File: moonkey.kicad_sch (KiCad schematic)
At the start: 35 parts, among them SW1 SW_Push, SW10 SW_Push, SW11 SW_Push, SW12 SW_Push, SW13 SW_Push, SW14 SW_Push, SW15 SW_Push, SW16 SW_Push, SW17 SW_Push, SW2 SW_Push, SW3 SW_Push, SW4 SW_Push, SW5 SW_Push, SW6 SW_Push, SW7 SW_Push, SW8 SW_Push, SW9 SW_Push

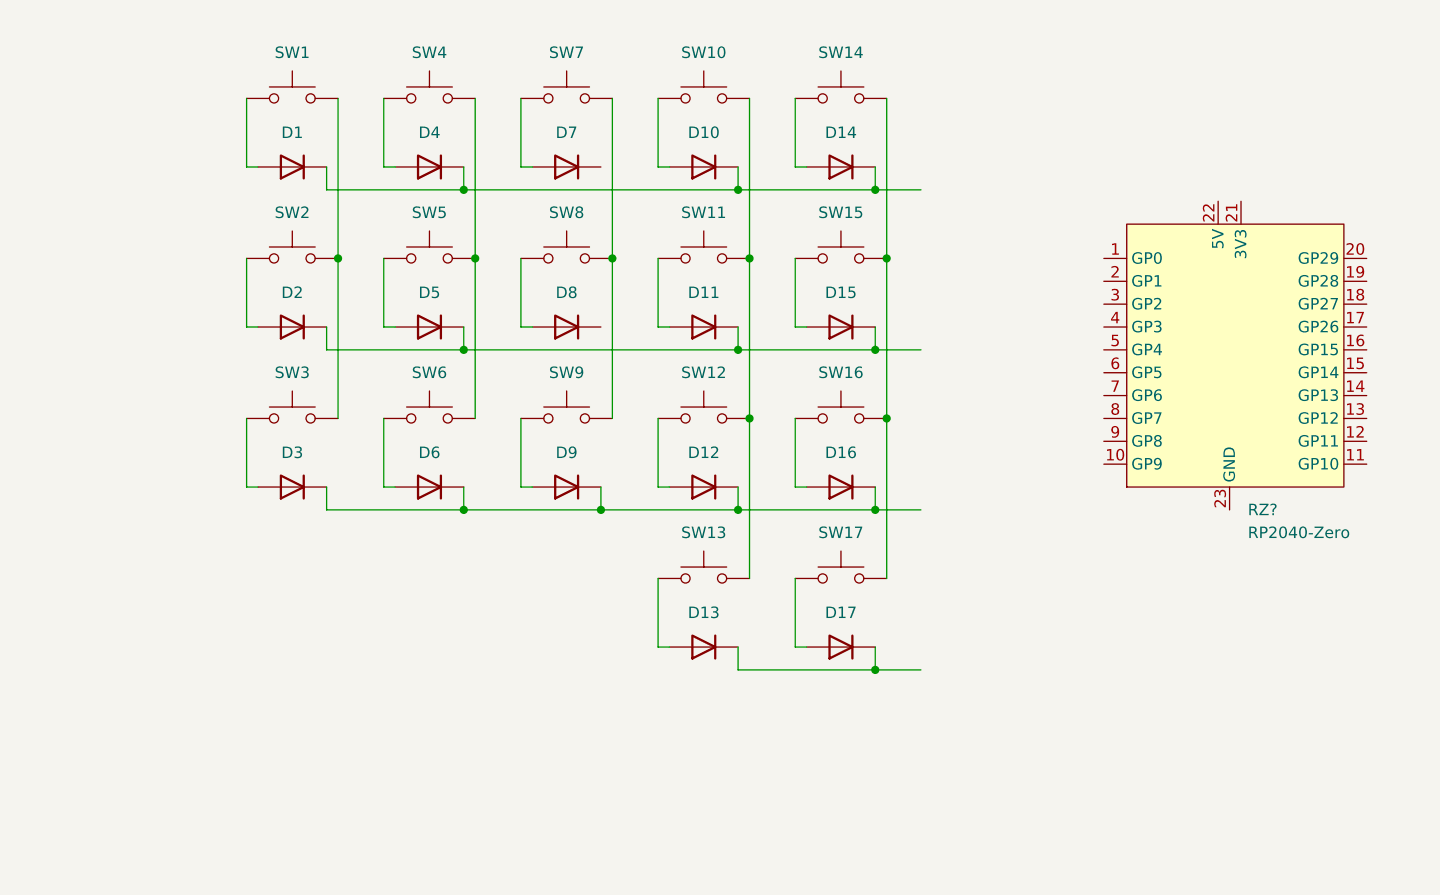
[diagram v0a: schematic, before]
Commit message: update
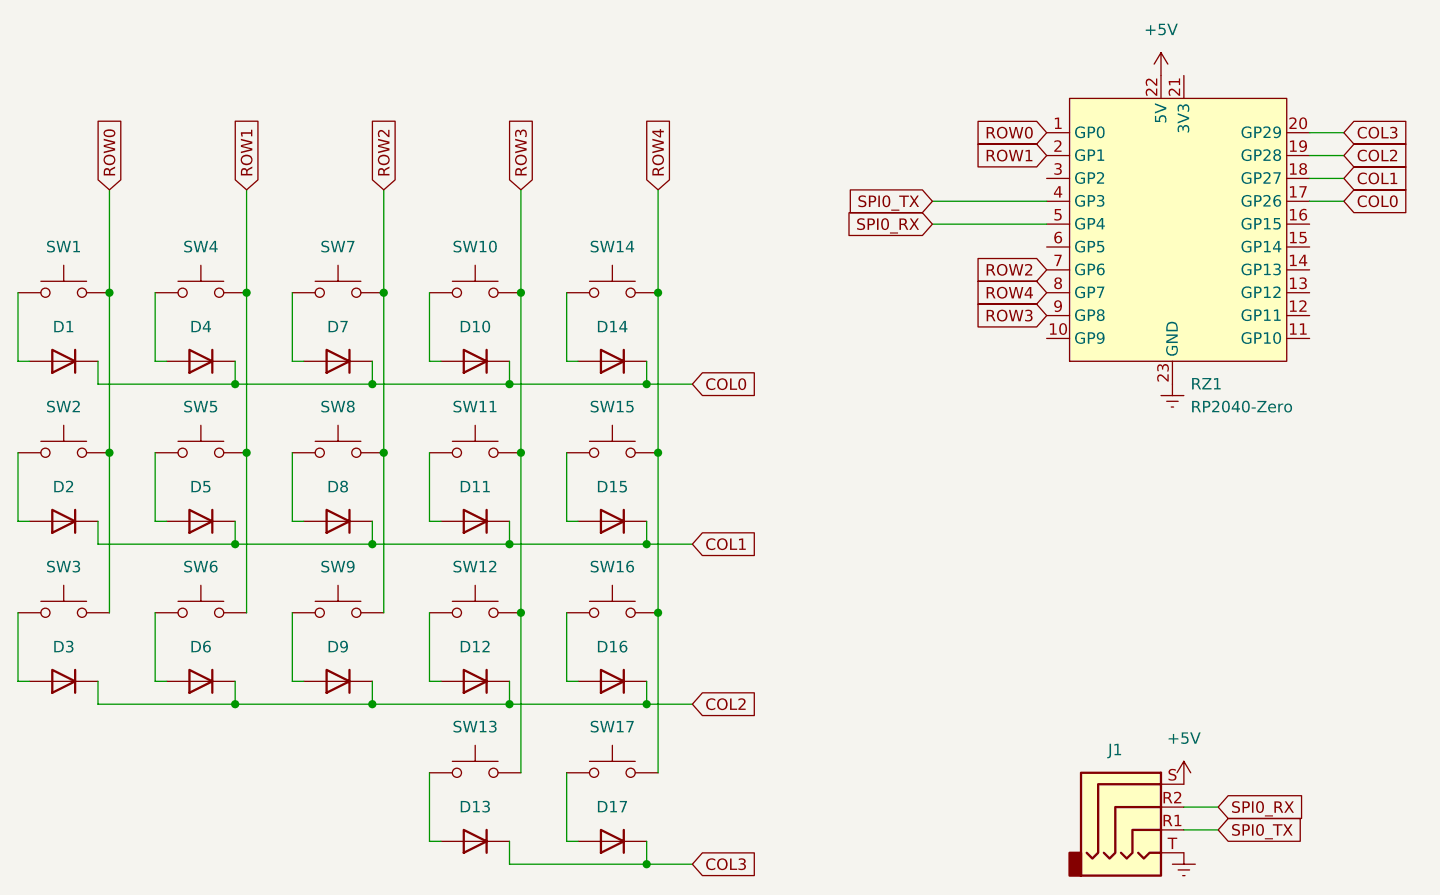
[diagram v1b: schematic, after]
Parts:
- added J1: AudioJack4, moonkey:PJ320A, symbol Connector:AudioJack4
- RZ1: renamed from RZ?; footprint (none) -> moonkey:RP2040
- SW1, SW10, SW11, SW12, SW13, SW14, SW15, SW16, SW17, SW2, SW3, SW4, SW5, SW6, SW7, SW8, SW9: footprint Switch_Keyboard_Cherry_MX:SW_Cherry_MX_PCB_1.00u -> moonkey:Cherry_1u_rev
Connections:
- net COL0: now reaches D1.1 (K), D10.1 (K), D14.1 (K), D4.1 (K)
- net COL0: now also D7.1 (K), RZ1.17 (GP26)
- net ROW4: now reaches SW14.2, SW15.2, SW16.2, SW17.2
- net ROW4: now also RZ1.8 (GP7)
- net COL2: now reaches D12.1 (K), D16.1 (K), D3.1 (K), D6.1 (K), D9.1 (K)
- net COL2: now also RZ1.19 (GP28)
- net ROW0: now reaches SW1.2, SW2.2, SW3.2
- net ROW0: now also RZ1.1 (GP0)
- net ROW2: now reaches SW7.2, SW8.2, SW9.2
- net ROW2: now also RZ1.7 (GP6)
- net COL1: now reaches RZ1.18 (GP27)
- net COL1: now also D11.1 (K), D15.1 (K), D2.1 (K), D5.1 (K), D8.1 (K)
- net ROW1: now reaches RZ1.2 (GP1)
- net ROW1: now also SW4.2, SW5.2, SW6.2
- net COL3: now reaches RZ1.20 (GP29)
- net COL3: now also D13.1 (K), D17.1 (K)
- net +5V: now reaches RZ1.22 (5V)
- net +5V: now also J1.S
- net Earth: now reaches RZ1.23 (GND)
- net Earth: now also J1.T
- net SPI0_TX: now reaches RZ1.4 (GP3)
- net SPI0_TX: now also J1.R1
- net SPI0_RX: now reaches RZ1.5 (GP4)
- net SPI0_RX: now also J1.R2
- net ROW3: now reaches RZ1.9 (GP8)
- net ROW3: now also SW10.2, SW11.2, SW12.2, SW13.2
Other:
- moved on the sheet: D1, D10, D11, D12, D13, D14, D15, D16, D17, D2, D3, D4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
